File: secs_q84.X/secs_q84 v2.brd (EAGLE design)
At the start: 78.4 x 58.4 mm, 54 parts, among them IC1 MAX203ECWP, IC4 PIC18F47Q84-I_PT

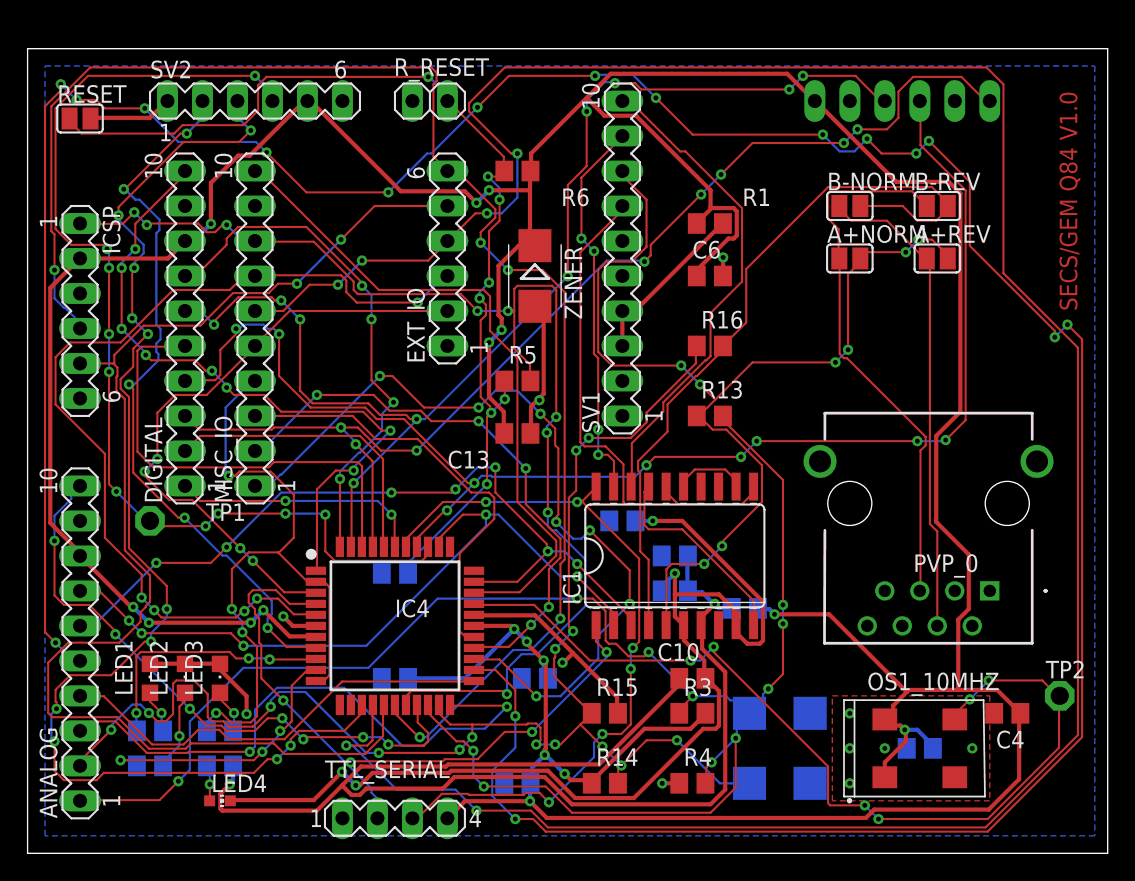
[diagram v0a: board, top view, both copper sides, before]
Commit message: up
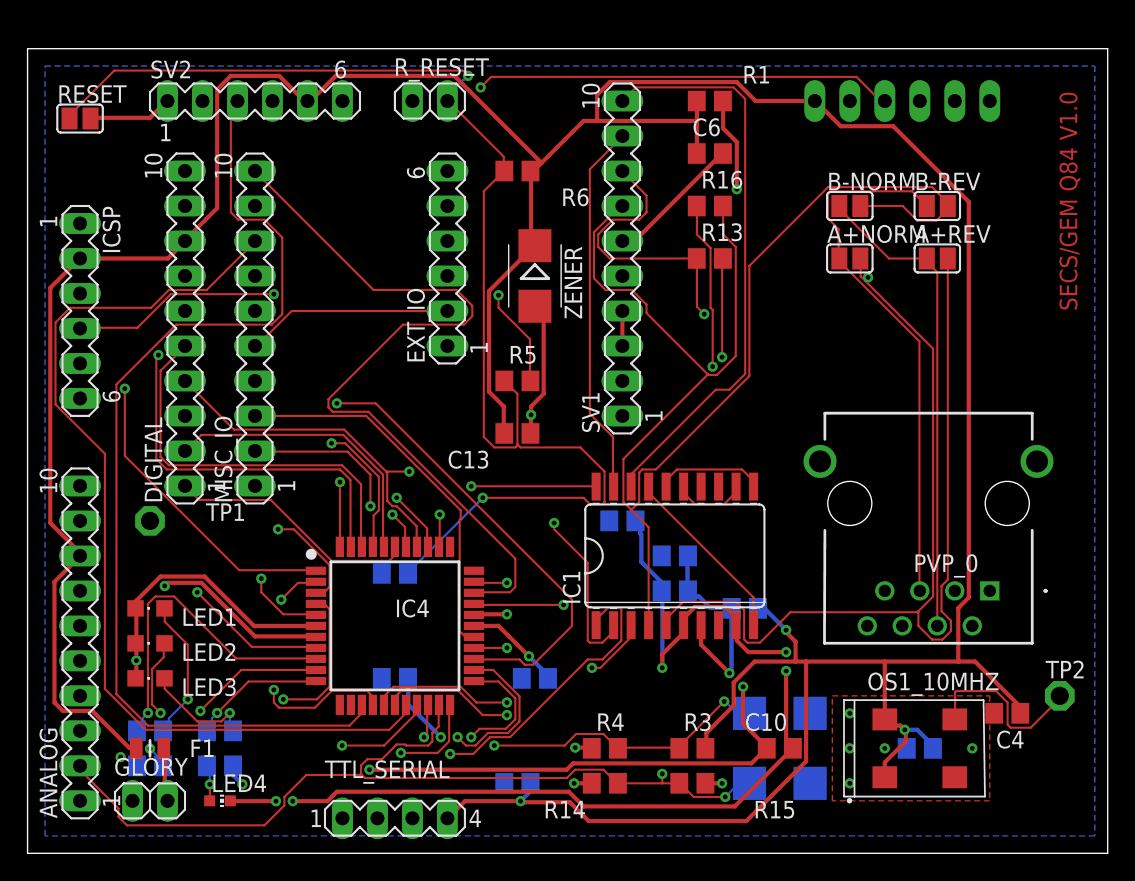
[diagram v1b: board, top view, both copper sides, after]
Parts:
- added F1: 0805L075WR, 0805L075WR:FUSC2114X125N
- added GLORY: GLORY, pinhead:1X02
- moved R13 11.4 mm to (71.1, 64.8)
- moved R16 10.2 mm to (71.1, 68.6)
- moved C6 8.89 mm to (71.1, 72.4)
- moved R1 8.89 mm to (71.1, 76.2)
- moved C10 8.13 mm to (76.2, 29.2)
- moved R15 8.13 mm to (69.8, 26.7)
- moved R4 6.84 mm to (63.5, 29.2)
- moved LED3 5.08 mm to (30.5, 34.3), turned to 90 degrees
- moved LED1 5.08 mm to (30.5, 39.4), turned to 90 degrees
- moved LED2 3.59 mm to (30.5, 36.8), turned to 90 degrees
- moved R3 2.54 mm to (69.8, 29.2)
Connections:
- new net POWERIN: F1.1, GLORY.2
- net VDD: now also F1.2
- net VSS: now also GLORY.1
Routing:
- net AN5: track 225.4 -> 41.2 mm, vias 17 -> 1
- net RB5: track 183.9 -> 55.7 mm, vias 6 -> 1
- net RS232TX: track 75.9 -> 116.4 mm, vias 8 -> 2
- net VCC: track 91.9 -> 62.8 mm, vias 2 -> 4
- net AN1: track 125.6 -> 98.2 mm, vias 11 -> 4
- net PGD: track 109.9 -> 84.4 mm, vias 5 -> 2
- net SCK1: track 99.2 -> 73.7 mm, vias 9 -> 1
- net RD7: track 67.4 -> 43.3 mm, vias 5 -> 1
- net MCLR_SIG: track 88.4 -> 109.9 mm, vias 9 -> 1
- net RS232RX: track 80.9 -> 99.8 mm
- net RELAY: track 60.6 -> 41.8 mm, vias 7 -> 1
- net R_RESET: track 75.7 -> 94.0 mm, vias 8 -> 2
- net CANTX: track 90.4 -> 74.7 mm, vias 11 -> 0
- net AN4: track 32.5 -> 48.0 mm, vias 0 -> 1
- net PC_RX2: track 54.1 -> 41.1 mm, vias 6 -> 2
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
